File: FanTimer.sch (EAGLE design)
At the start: 22 parts, among them IC2 NE555, T1 BT138-H

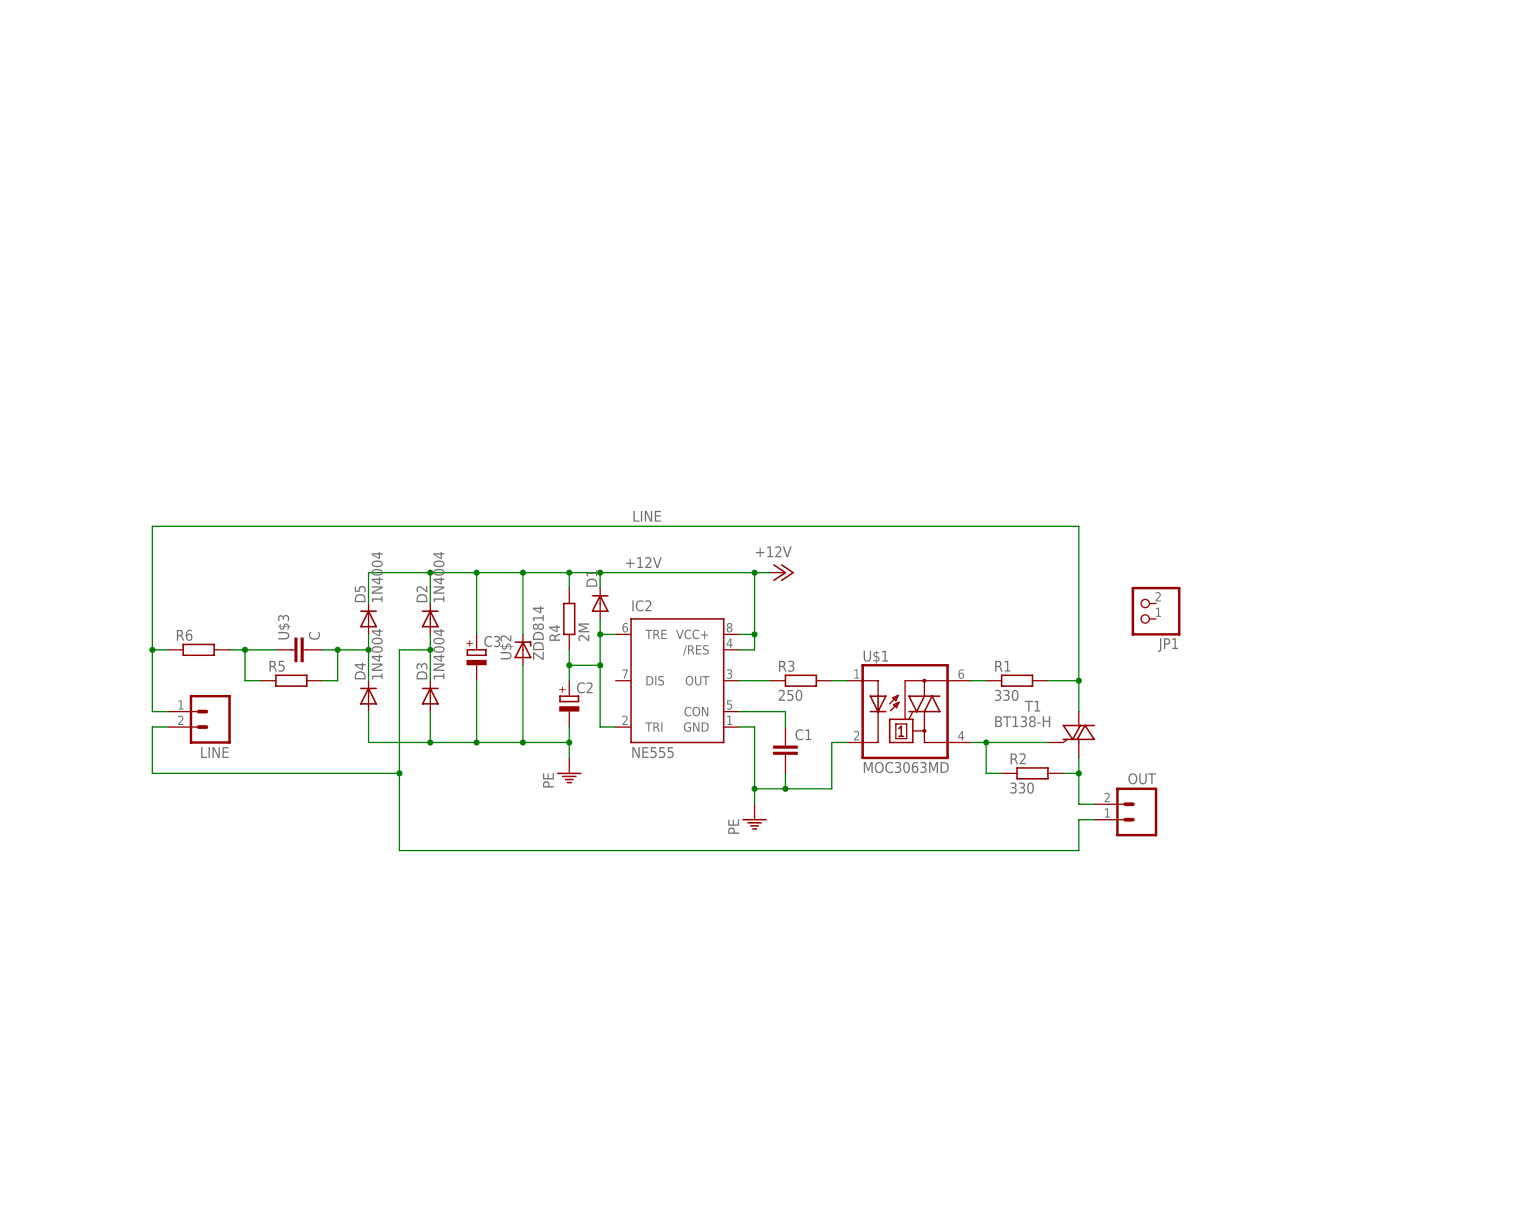
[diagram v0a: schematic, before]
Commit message: del 817
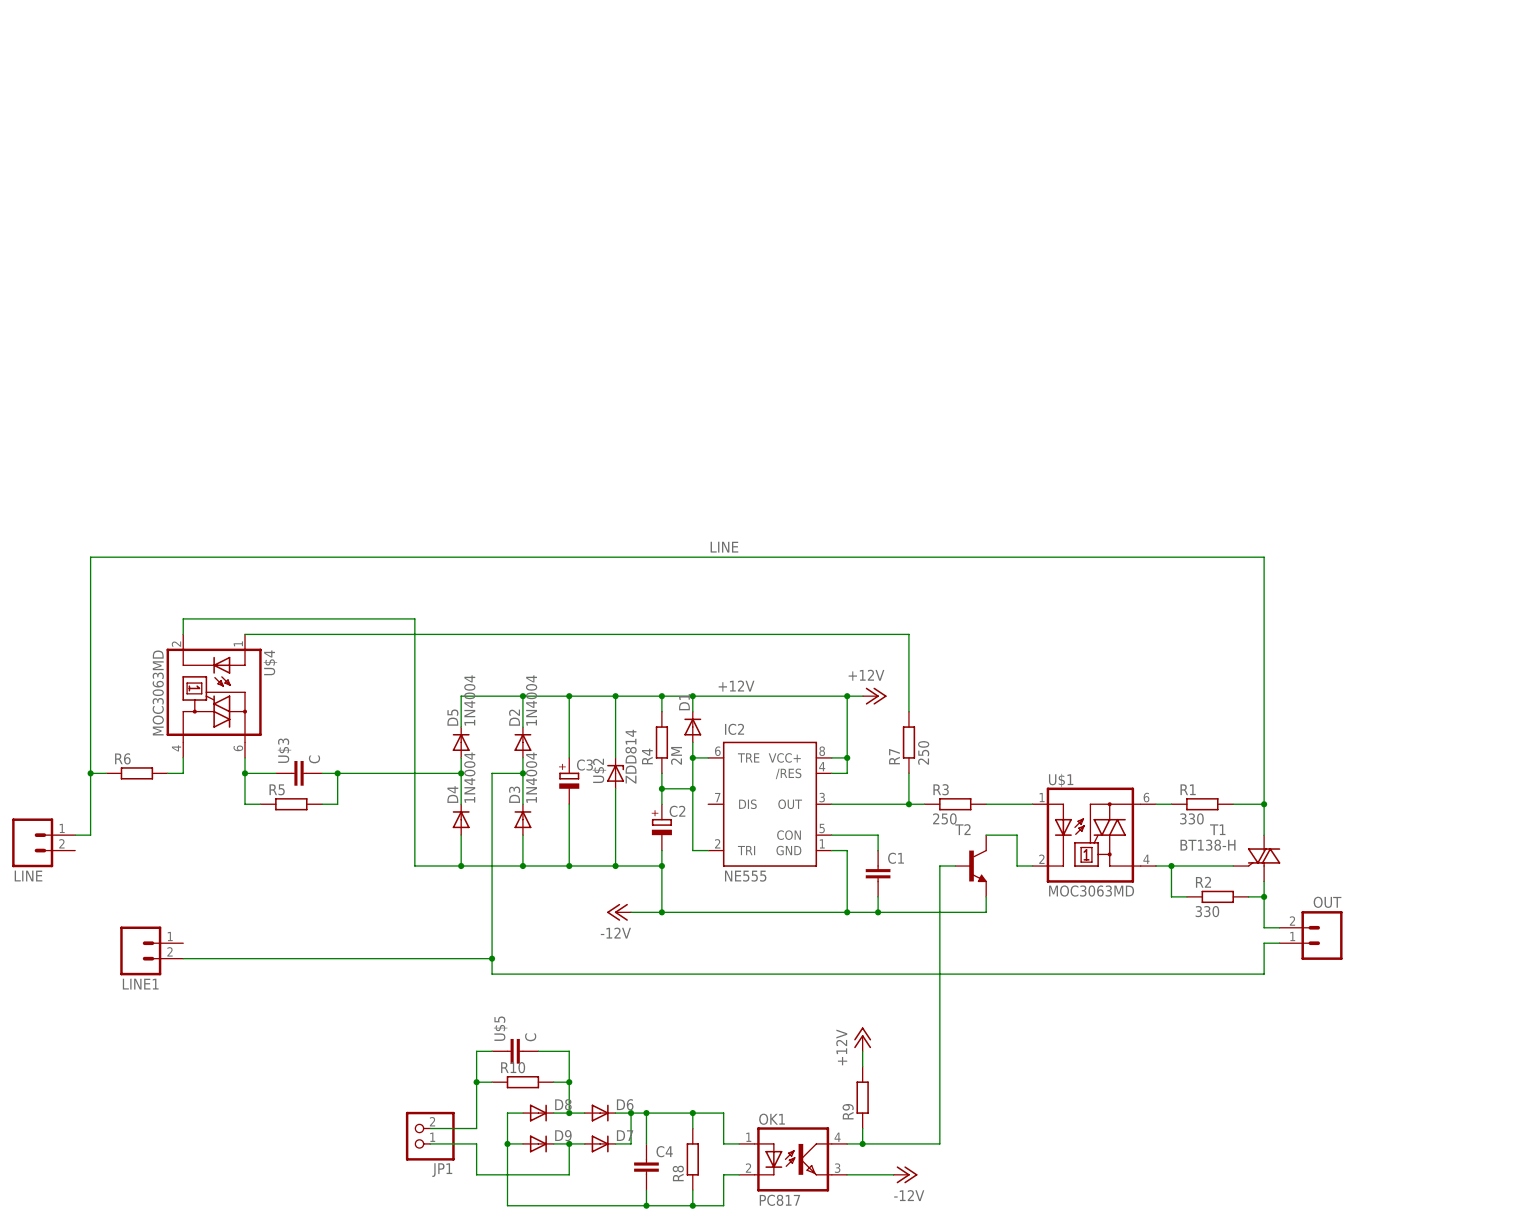
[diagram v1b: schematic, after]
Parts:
- added C4: (no value), rcl:C-EUC0805
- added D6, D7, D8, D9: (no value), diode:DIODE-SOD80C
- added LINE1: CON_2P, DSS0:CON_2P
- added OK1: PC817, optocoupler:PC817
- added R10: (no value), rcl:R-EU_0411/12
- added R7: 250, rcl:R-EU_0207/10
- added R8, R9: (no value), rcl:R-EU_R0805
- added T2: (no value), transistor:-NPN-TO92-ECB
- added U$4: MOC3063MD, DSS0:MOC3063MD
- added U$5: C, DSS0:C
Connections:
- removed net PE: C1.2, C2.-, C3.-, D3.A, D4.A, IC2.GND, U$1.C, U$2.A
- new net -12V: C1.2, C2.-, C3.-, D3.A, D4.A, IC2.GND, OK1.EMIT, T2.E, U$2.A, U$4.C
- new net N$1: T2.C, U$1.C
- new net N$10: C4.2, D8.A, D9.A, OK1.C, R8.1
- new net N$15: OK1.COL, R9.1, T2.B
- new net N$16: D6.A, D8.C, R10.2, U$5.2
- new net N$17: JP1.2, R10.1, U$5.1
- new net N$2: R6.2, U$4.A1
- new net N$21: D7.A, D9.C, JP1.1
- new net N$22: C4.1, D6.C, D7.C, OK1.A, R8.2
- new net N$4: R7.2, U$4.A
- net +12V: now also R9.2
- net N$11: now also LINE1.2; no longer LINE.2
- net N$12: now also R7.1
- net N$18: now also U$4.A2; no longer R6.2
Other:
- moved on the sheet: C1, C2, C3, D1, D2, D3, D4, D5, IC2, JP1, LINE, OUT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

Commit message: r1
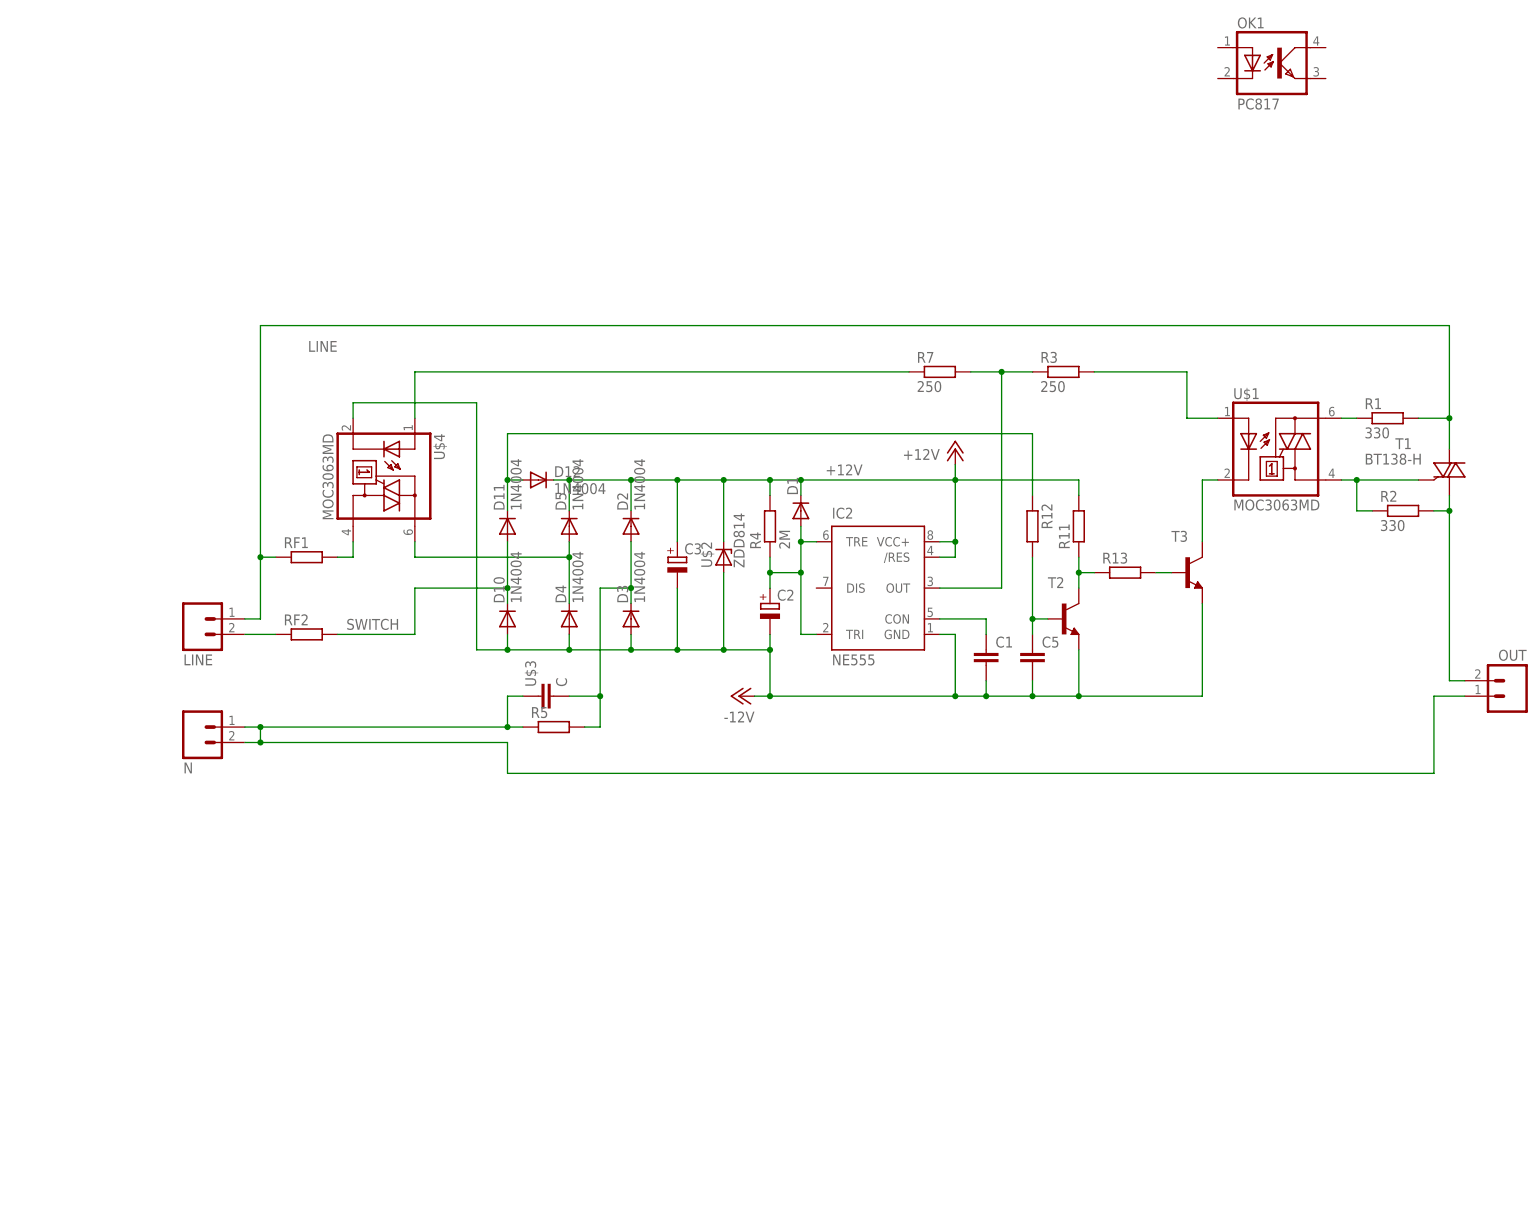
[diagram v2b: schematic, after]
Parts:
- removed C4: (no value), rcl:C-EUC0805
- removed D6, D7, D8, D9: (no value), diode:DIODE-SOD80C
- removed JP1: (no value), pinhead:PINHD-1X2
- removed LINE1: CON_2P, DSS0:CON_2P
- removed R10: (no value), rcl:R-EU_0411/12
- removed R6: (no value), rcl:R-EU_R1206
- removed R8, R9: (no value), rcl:R-EU_R0805
- removed U$5: C, DSS0:C
- added C5: (no value), rcl:C-EUC0805
- added D10, D11, D12: 1N4004, diode:1N4004
- added N: CON_2P, DSS0:CON_2P
- added R11, R12, R13: (no value), rcl:R-EU_0207/10
- added RF1, RF2: (no value), rcl:R-EU_R1206
- added T3: (no value), transistor:-NPN-TO92-ECB
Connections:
- removed net N$10: C4.2, D8.A, D9.A, OK1.C, R8.1
- removed net N$11: D2.A, D3.C, LINE1.2, OUT.1
- removed net N$15: OK1.COL, R9.1, T2.B
- removed net N$16: D6.A, D8.C, R10.2, U$5.2
- removed net N$17: JP1.2, R10.1, U$5.1
- removed net N$21: D7.A, D9.C, JP1.1
- removed net N$22: C4.1, D6.C, D7.C, OK1.A, R8.2
- new net N$20: D2.A, D3.C, R5.2, U$3.2
- new net N$23: R13.2, T3.B
- new net N$24: N.1, N.2, OUT.1, R5.1, U$3.1
- new net N$26: C5.1, R12.2, T2.B
- new net N$28: T3.C, U$1.C
- new net N$7: D11.C, D12.A, R12.1
- new net SWITCH: D10.C, D11.A, RF2.2
- net +12V: now also D12.C, R11.2; no longer R9.2
- net -12V: now also C5.2, D10.A, T3.E; no longer OK1.EMIT
- net LINE: now also RF1.1; no longer R6.1
- net N$1: now also D4.C, D5.A, U$4.A2; no longer T2.C, U$1.C
- net N$12: now also R7.2; no longer R7.1
- net N$14: now also R11.1, R13.1, T2.C; no longer D4.C, D5.A, R5.2, U$3.2
- net N$18: now also LINE.2, RF2.1; no longer R5.1, U$3.1, U$4.A2
- net N$2: now also RF1.2; no longer R6.2
- net N$4: now also R7.1; no longer R7.2
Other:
- moved on the sheet: C1, C2, C3, D1, D2, D3, D4, D5, IC2, LINE, OK1, OUT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

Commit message: .
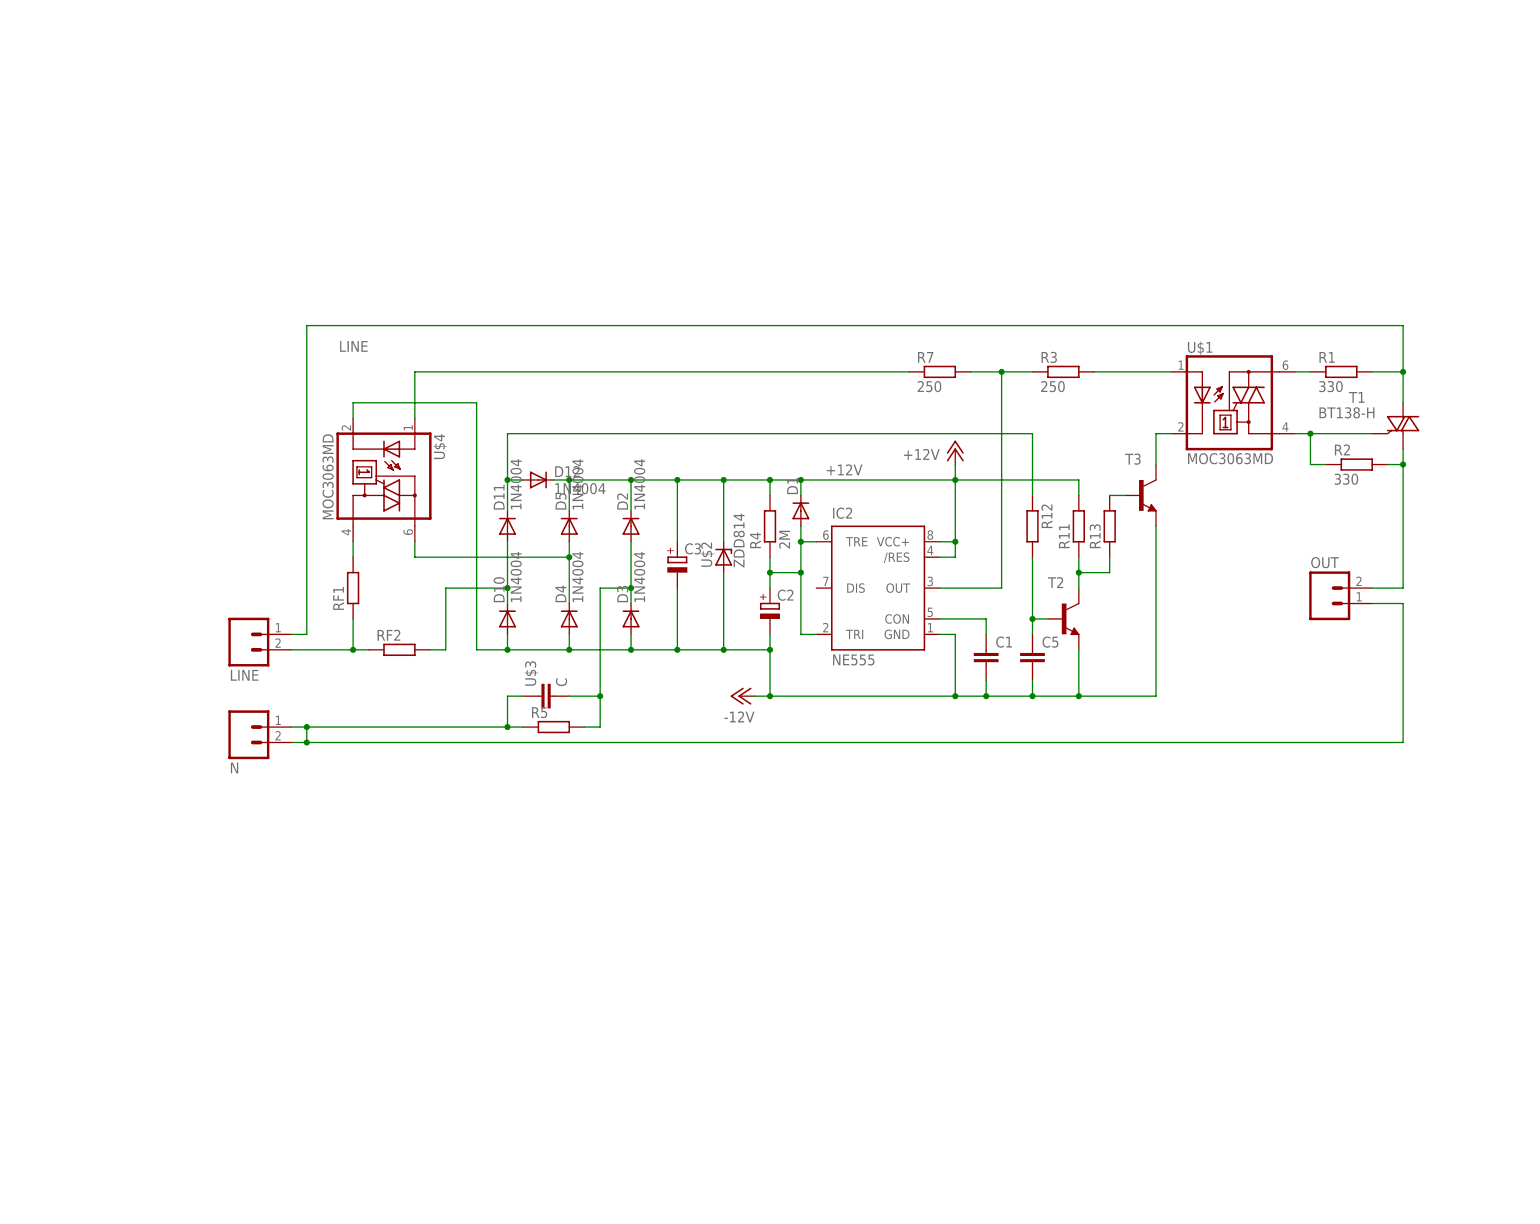
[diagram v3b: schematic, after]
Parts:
- removed OK1: PC817, optocoupler:PC817
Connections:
- net LINE: no longer RF1.1
- net N$18: now also RF1.1
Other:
- moved on the sheet: LINE, N, OUT, R1, R13, R2, RF1, RF2, T1, T3, U$1
